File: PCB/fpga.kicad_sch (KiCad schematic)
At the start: 16 parts, among them IC1 S25FL256LAGMFI003, J1 0878311420, J4 62684-402100ALF, U4 XC7A100T-FTG256, U5 IS62C1024AL-35QLI-TR, Y2 ECS-3953M-400-BN-TR

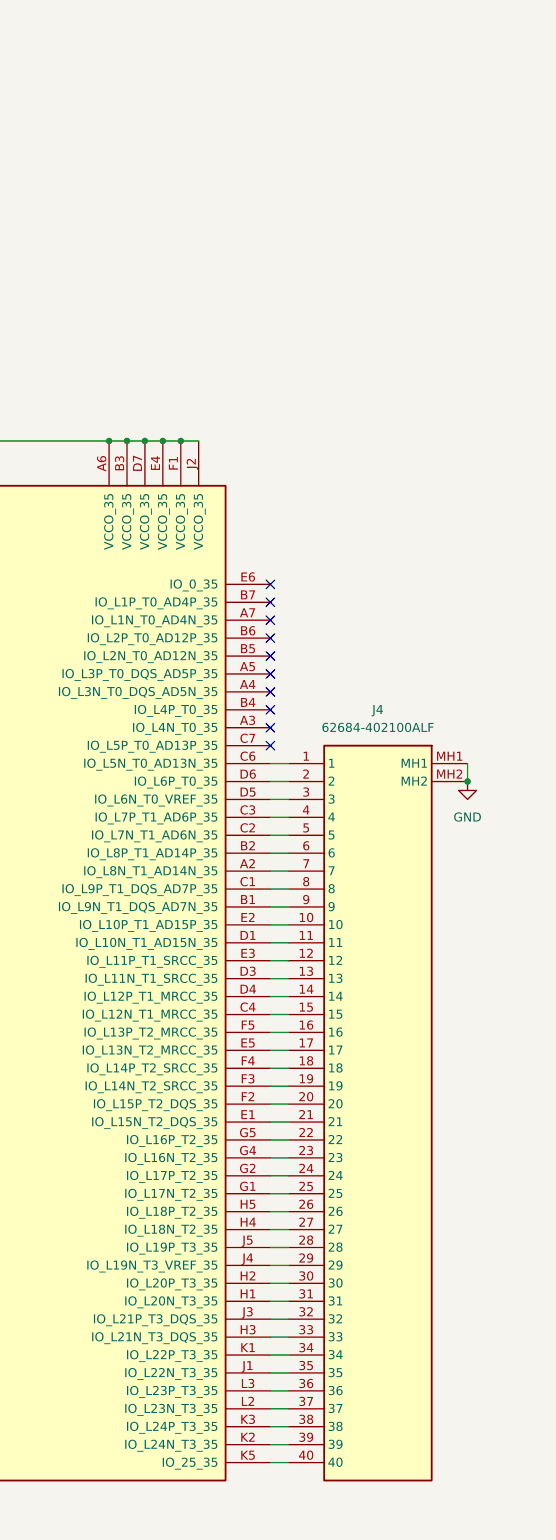
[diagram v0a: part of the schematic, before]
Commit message: PCB
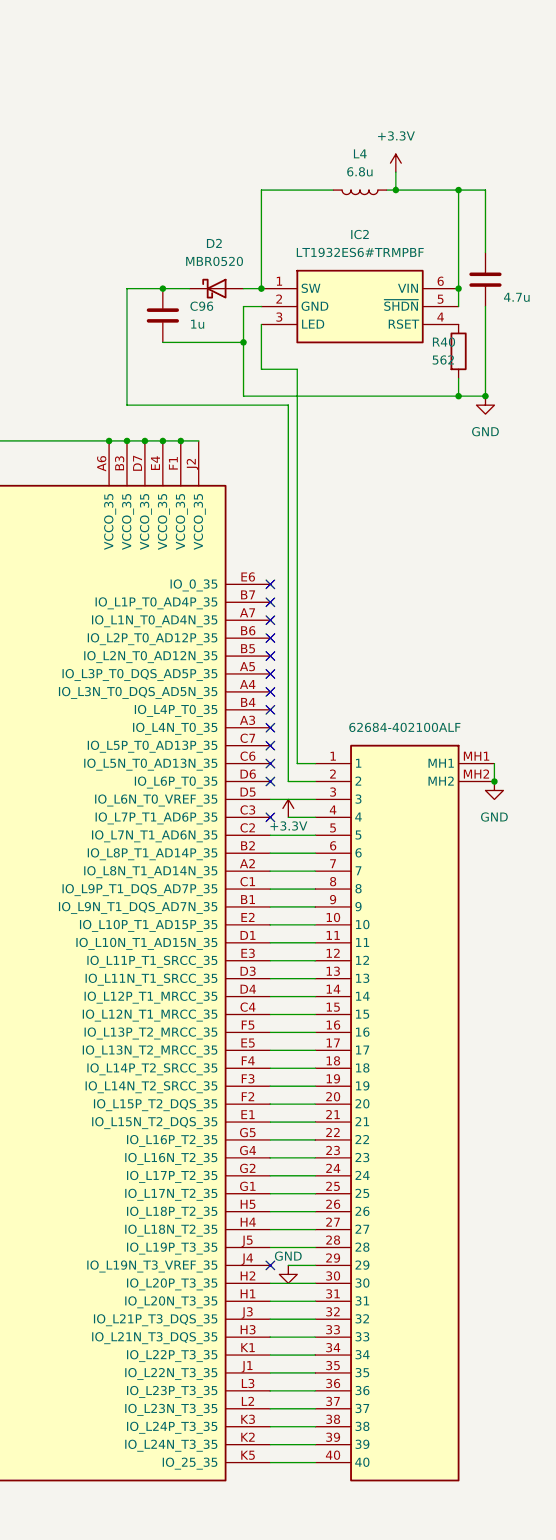
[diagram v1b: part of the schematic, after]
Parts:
- added C95: 4.7u, Capacitor_SMD:C_0805_2012Metric_Pad1.18x1.45mm_HandSolder, symbol Device:C
- added C96: 1u, Capacitor_SMD:C_0805_2012Metric_Pad1.18x1.45mm_HandSolder, symbol Device:C
- added D2: MBR0520, Diode_SMD:D_SOD-123, symbol Diode:MBR0520
- added IC2: LT1932ES6#TRMPBF, ledDriver:SOT95P280X100-6N, symbol LT1932ES6#TRMPBF:LT1932ES6#TRMPBF
- added L4: 6.8u, Inductor_SMD:L_0805_2012Metric_Pad1.05x1.20mm_HandSolder, symbol Device:L
- added R40: 562, Resistor_SMD:R_0805_2012Metric_Pad1.20x1.40mm_HandSolder, symbol Device:R
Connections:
- net +3.3V: now also J4.4, C95.1, IC2.5 (~{SHDN}), IC2.6 (VIN), L4.1
- net GND: now also J4.29, C95.2, C96.2, IC2.2 (GND), R40.2
- net at J4.1: now also IC2.3 (LED); no longer U4.C6 (IO_L5N_T0_AD13N_35)
- net at J4.2: now also C96.1, D2.1 (K); no longer U4.D6 (IO_L6P_T0_35)
- net at U4.J4 (IO_L19N_T3_VREF_35): no longer J4.29
- net at U4.C3 (IO_L7P_T1_AD6P_35): no longer J4.4
- new net: IC2.4 (RSET), R40.1
- new net: D2.2 (A), IC2.1 (SW), L4.2
- no-connect marks 77 -> 81
